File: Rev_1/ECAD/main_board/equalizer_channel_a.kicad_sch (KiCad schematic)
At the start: 24 parts, among them U20 NE5532, U21 NE5532

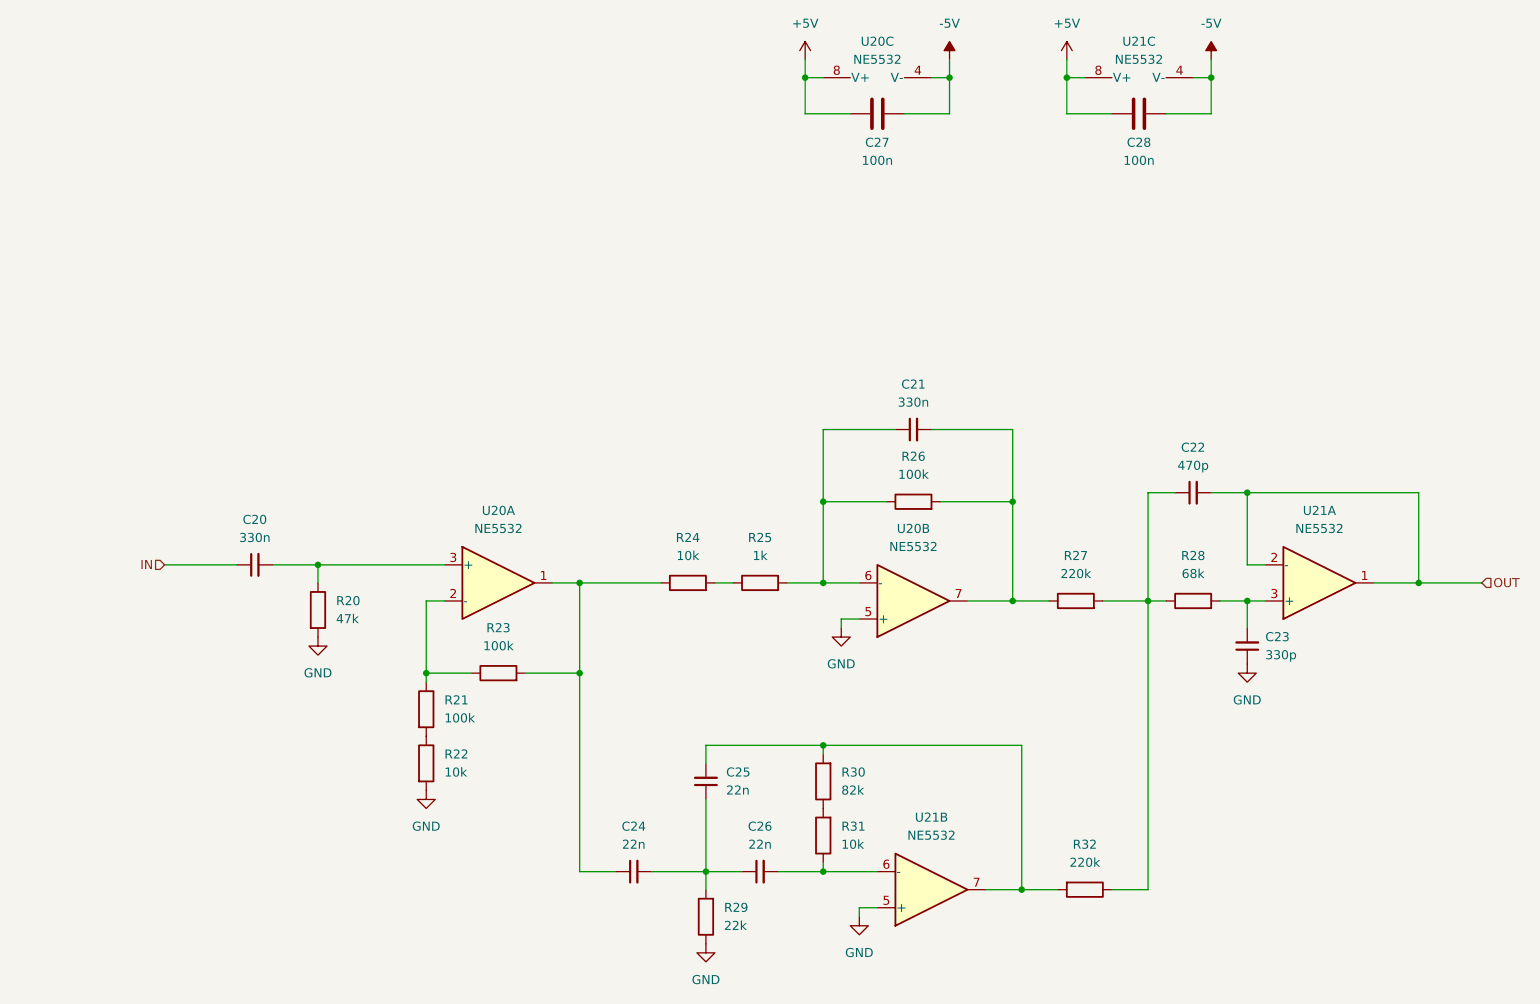
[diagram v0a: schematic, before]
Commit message: Semi finsihed schematic
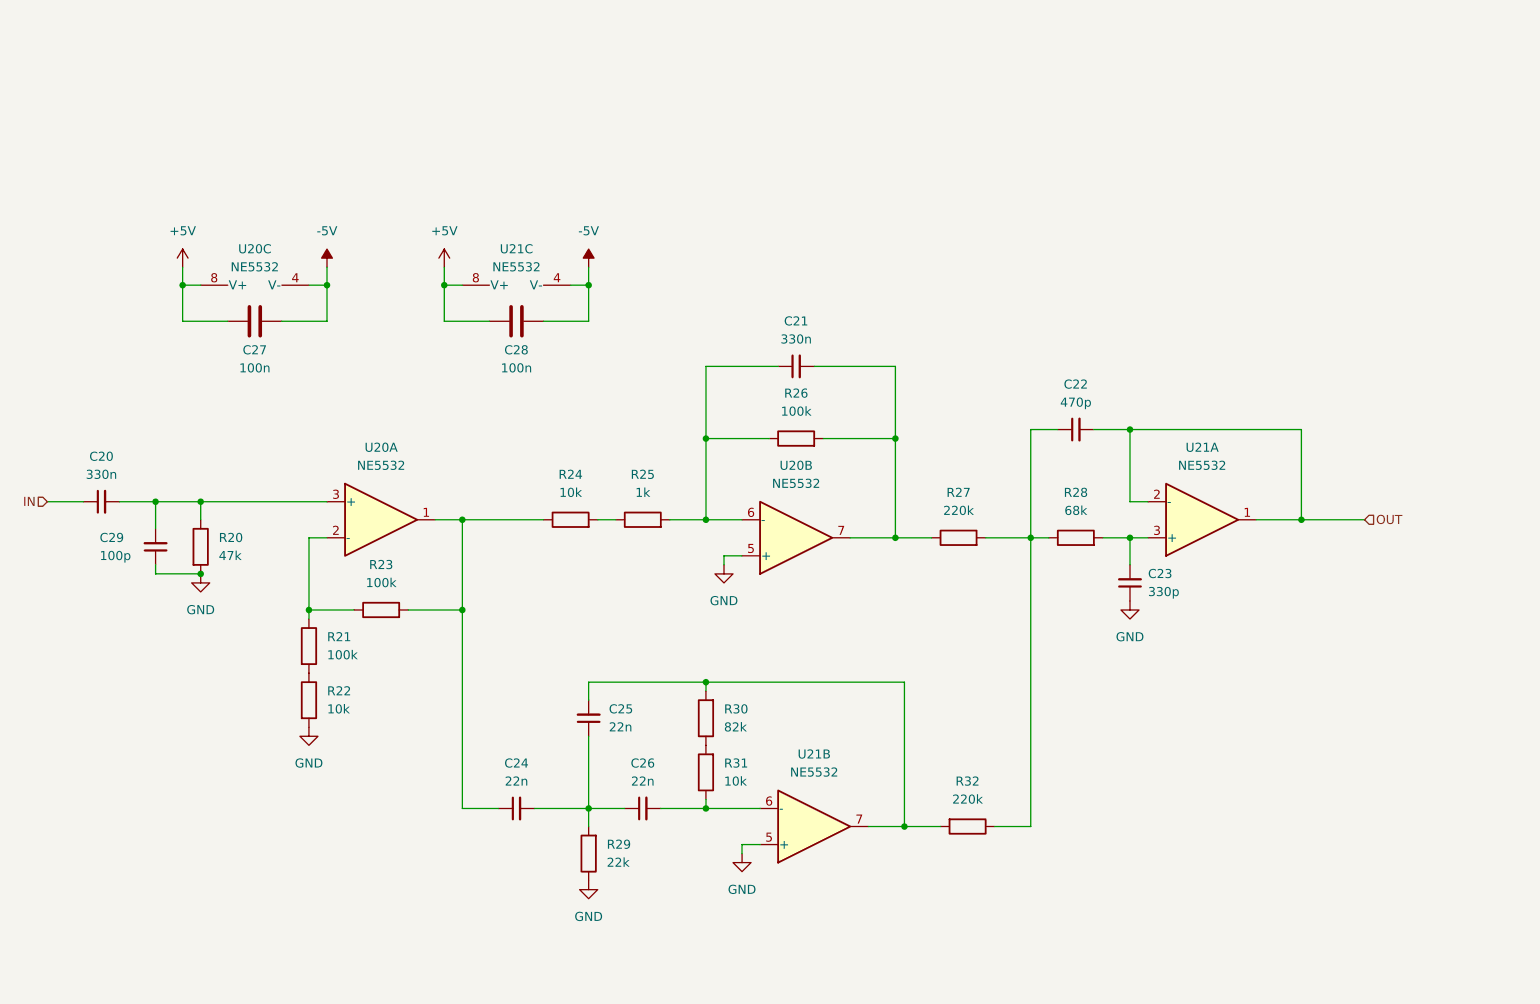
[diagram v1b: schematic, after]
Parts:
- added C29: 100p, Capacitor_SMD:C_0805_2012Metric, symbol Device:C_Small
- C20, C21, C22, C23, C24, C25, C26, C27, C28: footprint (none) -> Capacitor_SMD:C_0805_2012Metric
- R20, R21, R22, R23, R24, R25, R26, R27, R28, R29, R30, R31, R32: footprint (none) -> Resistor_SMD:R_0805_2012Metric
- U20, U21: footprint (none) -> Package_SO:SOIC-8_5.3x6.2mm_P1.27mm
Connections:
- net GND: now also C29.1
- net at C20.2, R20.1, U20.3 (+): now also C29.2
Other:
- moved on the sheet: C20, C21, C22, C23, C24, C25, C26, C27, C28, R20, R21, R22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
